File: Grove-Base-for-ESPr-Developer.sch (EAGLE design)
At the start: 8 parts, among them J1 4P-2.0, J2 4P-2.0, J3 4P-2.0, J4 4P-2.0

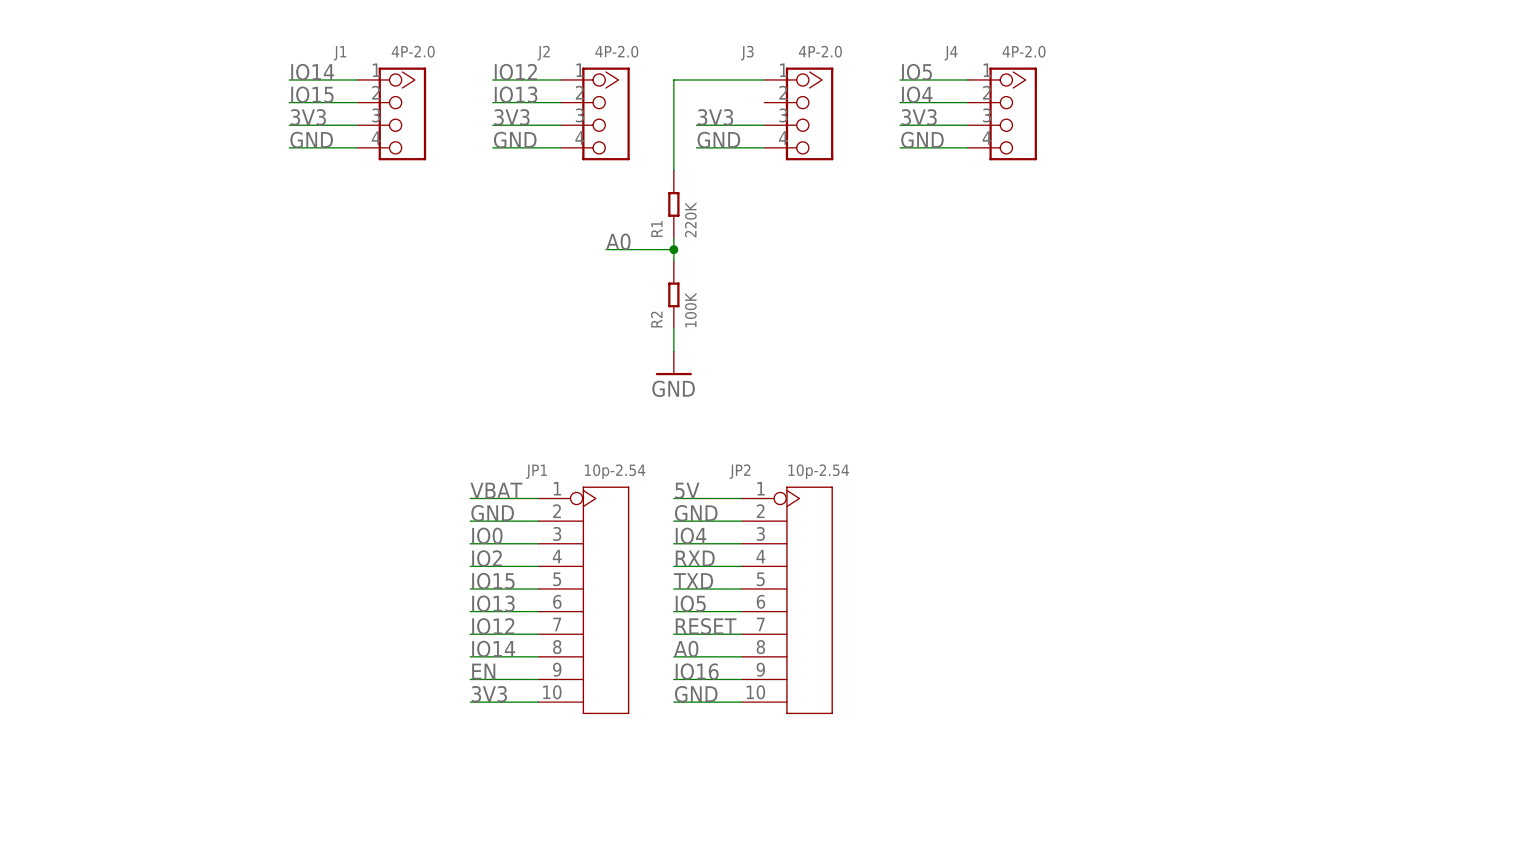
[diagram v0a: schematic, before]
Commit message: 1st 5V evt
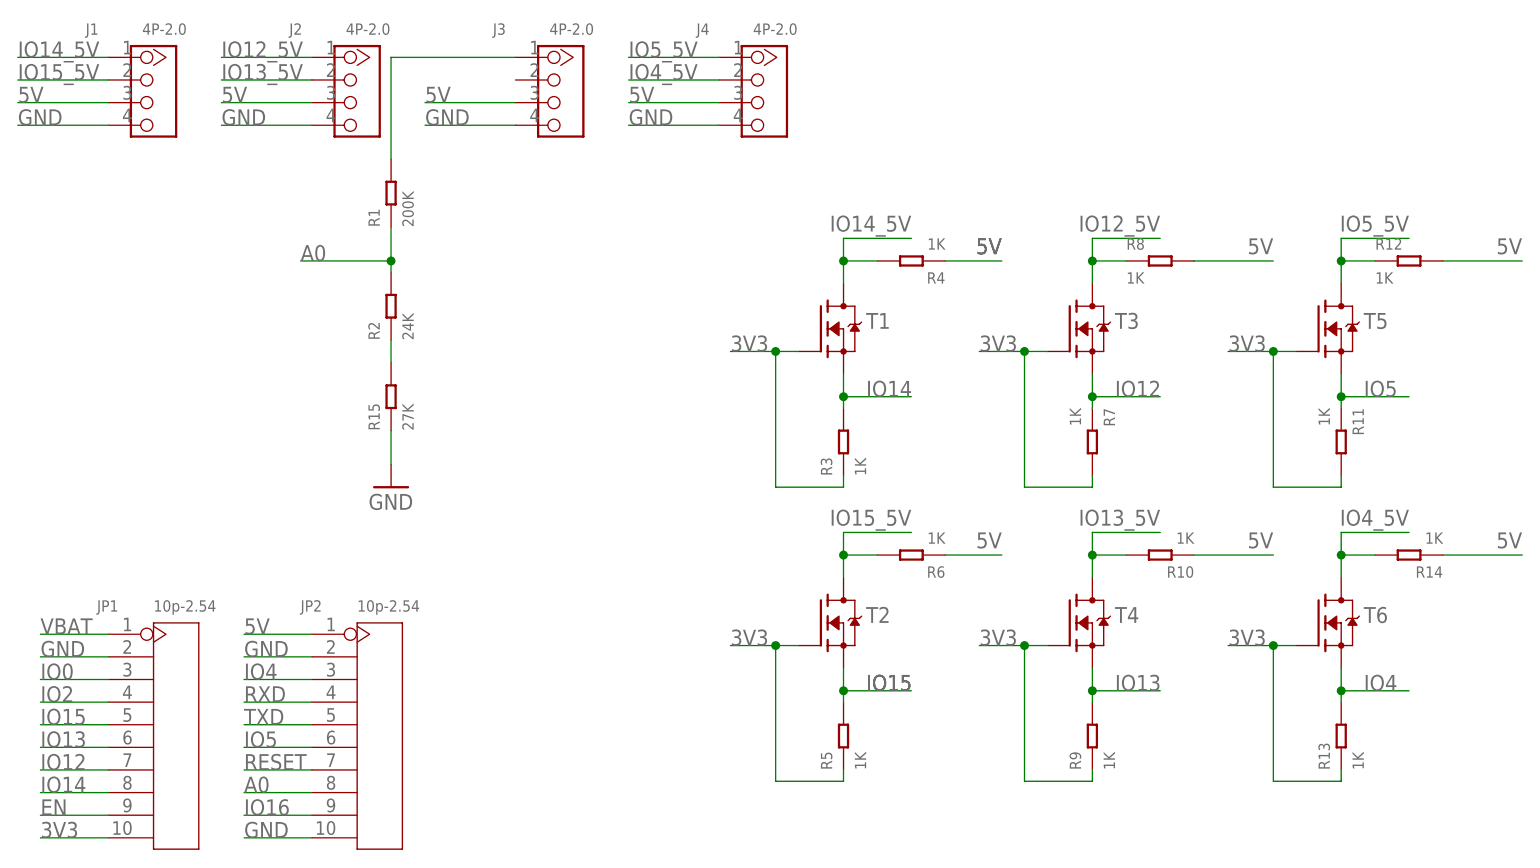
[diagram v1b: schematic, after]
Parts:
- added R10, R11, R12, R13, R14, R3, R4, R5, R6, R7, R8, R9: 1K, Seeed-OPL-Resistor:SMD-RES-220K-1%-1/10W(0603)
- added R15: 27K, Seeed-OPL-Resistor:SMD-RES-100K-1%-1/10W(0603)
- added T1, T2, T3, T4, T5, T6: (no value), we-transistor:MOSFET-N-SOT23
- R1: value 220K -> 200K
- R2: value 100K -> 24K
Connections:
- new net IO12_5V: J2.1, R8.1, T3.D
- new net IO13_5V: J2.2, R10.2, T4.D
- new net IO14_5V: J1.1, R4.2, T1.D
- new net IO15_5V: J1.2, R6.2, T2.D
- new net IO4_5V: J4.2, R14.2, T6.D
- new net IO5_5V: J4.1, R12.1, T5.D
- new net N$6: R15.2, R2.1
- net 3V3: now also R11.2, R13.1, R3.1, R5.1, R7.2, R9.1, T1.G, T2.G, T3.G, T4.G, T5.G, T6.G; no longer J1.3, J2.3, J3.3, J4.3
- net 5V: now also J1.3, J2.3, J3.3, J4.3, R10.1, R12.2, R14.1, R4.1, R6.1, R8.2
- net GND: now also R15.1; no longer R2.1
- net IO12: now also R7.1, T3.S; no longer J2.1
- net IO13: now also R9.2, T4.S; no longer J2.2
- net IO14: now also R3.2, T1.S; no longer J1.1
- net IO15: now also R5.2, T2.S; no longer J1.2
- net IO4: now also R13.2, T6.S; no longer J4.2
- net IO5: now also R11.1, T5.S; no longer J4.1
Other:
- moved on the sheet: J1, J2, J3, J4, JP1, JP2, R1, R2
